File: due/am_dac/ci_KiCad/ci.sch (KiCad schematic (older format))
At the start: 18 parts, among them J1 Entrada do sinal de áudio

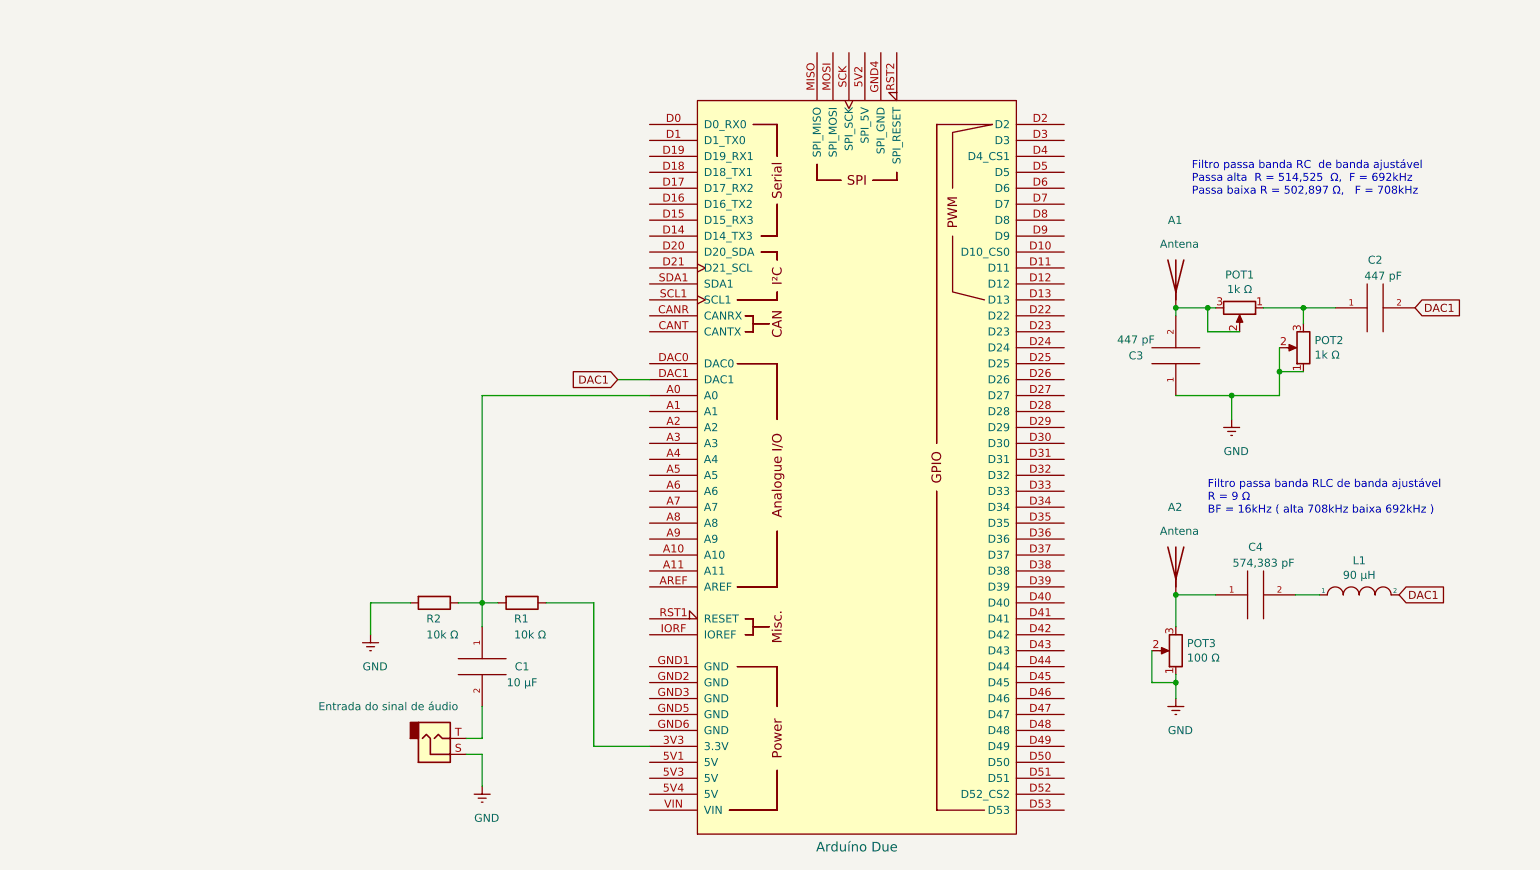
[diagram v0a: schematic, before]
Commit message: UP due am dac
Signed-off-by: fgl27 <fglfgl27@gmail.com>
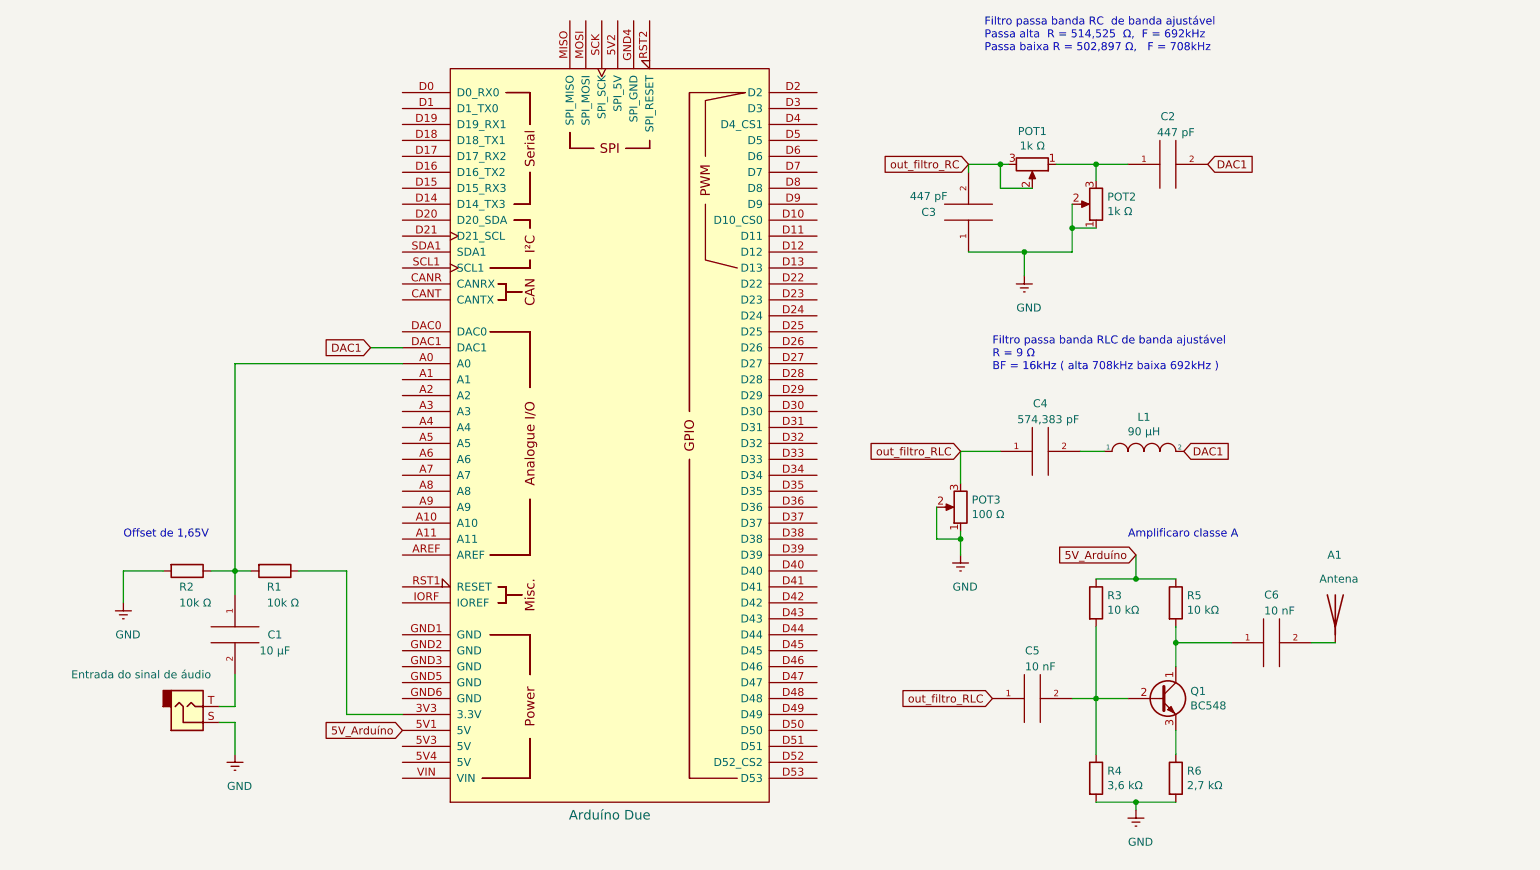
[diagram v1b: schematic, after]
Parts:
- removed A2: Antena, symbol Device:Antenna
- added C5, C6: 10 nF, symbol pspice:CAP
- added GND: GNDREF, symbol power:GNDREF
- added Q1: BC548, Package_TO_SOT_THT:TO-92_Inline, symbol Transistor_BJT:BC548
- added R3, R5: 10 kΩ, symbol Device:R
- added R4: 3,6 kΩ, symbol Device:R
- added R6: 2,7 kΩ, symbol Device:R
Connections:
- net GNDREF: now also GND.1 (GNDREF), R4.2, R6.2
- net out_filtro_RC: now reaches C3.2, POT1.2, POT1.3
- net out_filtro_RC: no longer A1.1 (A)
- net 5V_Arduíno: now reaches XA1.5V1 (5V)
- net 5V_Arduíno: now also R3.1, R5.1
- net out_filtro_RLC: now reaches C4.1, POT3.3
- net out_filtro_RLC: now also C5.1
- new net: A1.1 (A), C6.2
- new net: C6.1, Q1.1 (C), R5.2
- new net: C5.2, Q1.2 (B), R3.2, R4.1
- new net: Q1.3 (E), R6.1
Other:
- note added: "Amplificaro classe A"
- note added: "Offset de 1,65V"
- moved on the sheet: A1, C1, C2, C3, C4, L1, POT1, POT2, POT3, R1, R2
